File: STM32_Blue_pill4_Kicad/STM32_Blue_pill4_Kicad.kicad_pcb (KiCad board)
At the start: 2 copper layers, 28 parts, among them J1 USB_B_Micro, J3 Conn_01x04_Pin, J4 Conn_01x04_Pin, J5 Conn_01x04_Pin, SW1 SW_SPDT, U1 STM32F103C8T6, U3 AMS1117-3.3, Y1 Crystal_GND24

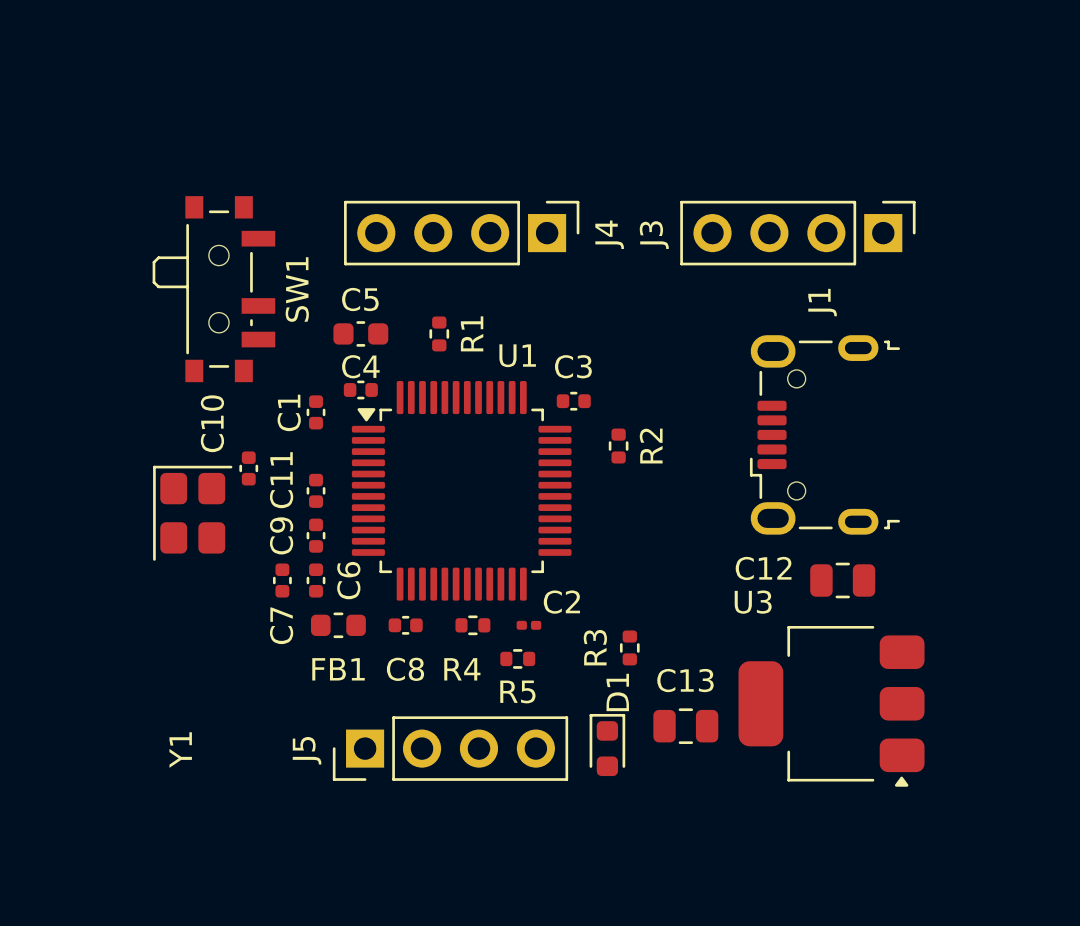
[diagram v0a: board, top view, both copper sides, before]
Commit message: Routing of STM32 Pill is finished
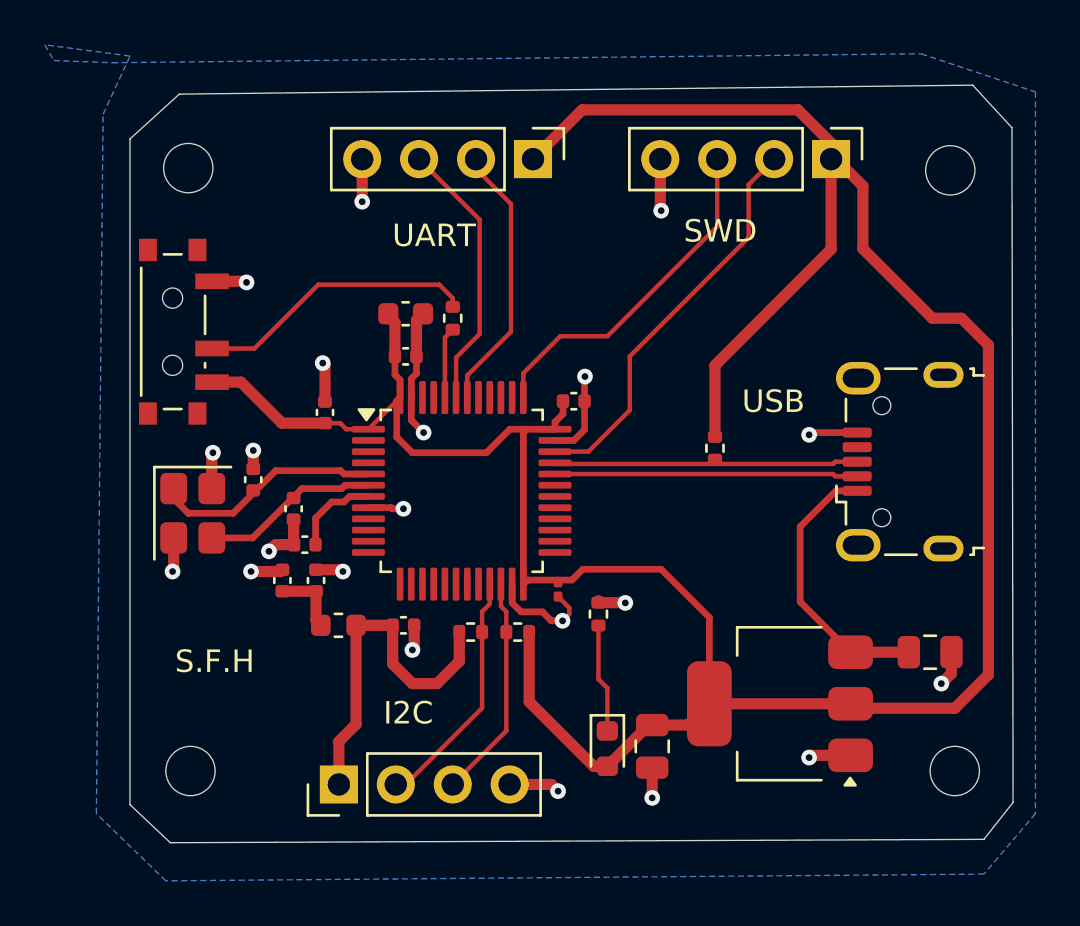
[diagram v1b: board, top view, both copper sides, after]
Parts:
- added H1: MountingHole, MountingHole:MountingHole_2.2mm_M2, F.Cu at (120.5, 111.0)
- added H2: MountingHole, MountingHole:MountingHole_2.2mm_M2, F.Cu at (120.3, 84.2)
- added H3: MountingHole, MountingHole:MountingHole_2.2mm_M2, F.Cu at (86.4, 111.0)
- added H4: MountingHole, MountingHole:MountingHole_2.2mm_M2, F.Cu at (86.3, 84.1)
- moved C12 5.04 mm to (119.4, 105.7), turned to 0 degrees
- moved R2 4.30 mm to (109.8, 96.6)
- moved J3 4.04 mm to (115.0, 83.7)
- moved J1 3.98 mm to (118.0, 97.2)
- moved J4 3.36 mm to (101.7, 83.7)
- moved SW1 2.81 mm to (85.9, 91.4)
- moved C4 2.50 mm to (96.0, 92.5), turned to 0 degrees
- moved U3 2.30 mm to (112.7, 108.0)
- moved C5 2.19 mm to (96.0, 90.6), turned to 0 degrees
- moved C2 2.06 mm to (102.8, 102.9), turned to -90 degrees
- moved R3 2.06 mm to (104.6, 104.0)
- moved J5 1.98 mm to (93.0, 111.6)
- moved C13 1.75 mm to (107.0, 109.9), turned to -90 degrees
- moved C11 1.28 mm to (91.0, 99.3)
- moved R5 1.20 mm to (101.0, 104.8)
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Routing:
- net +3.3V: track 0.00 -> 144.5 mm
- net GND: track 0.00 -> 44.4 mm, vias 0 -> 21
- net /SWDIO: track 0.00 -> 18.0 mm
- net /SWCLK: track 0.00 -> 15.5 mm
- net /USB_DM+: track 0.00 -> 13.5 mm
- net /USB_DM-: track 0.00 -> 13.5 mm
- net /BOOT0_SWITCH: track 0.00 -> 12.6 mm
- net VBUS: track 0.00 -> 12.3 mm
- net /USART1_RX: track 0.00 -> 12.2 mm
- net /USART1_TX: track 0.00 -> 12.1 mm
- net /12C_SCL: track 0.00 -> 10.9 mm
- net /HSE_IN: track 0.00 -> 10.7 mm
- net /12C_SDA: track 0.00 -> 10.0 mm
- net /HSE_OUT: track 0.00 -> 7.96 mm
- net Net-(D1-K): track 0.00 -> 4.87 mm
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- added copper zone on B.Cu, net GND
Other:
- board outline added: 39.4 x 33.8 mm
- board text added: "I2C"
- board text added: "S.F.H"
- board text added: "SWD"
- board text added: "UART"
- board text added: "USB"
